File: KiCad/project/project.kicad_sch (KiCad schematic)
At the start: 27 parts, among them P1 TerminalBlock 5P 5.0mm, U1 DRV8313PWPR

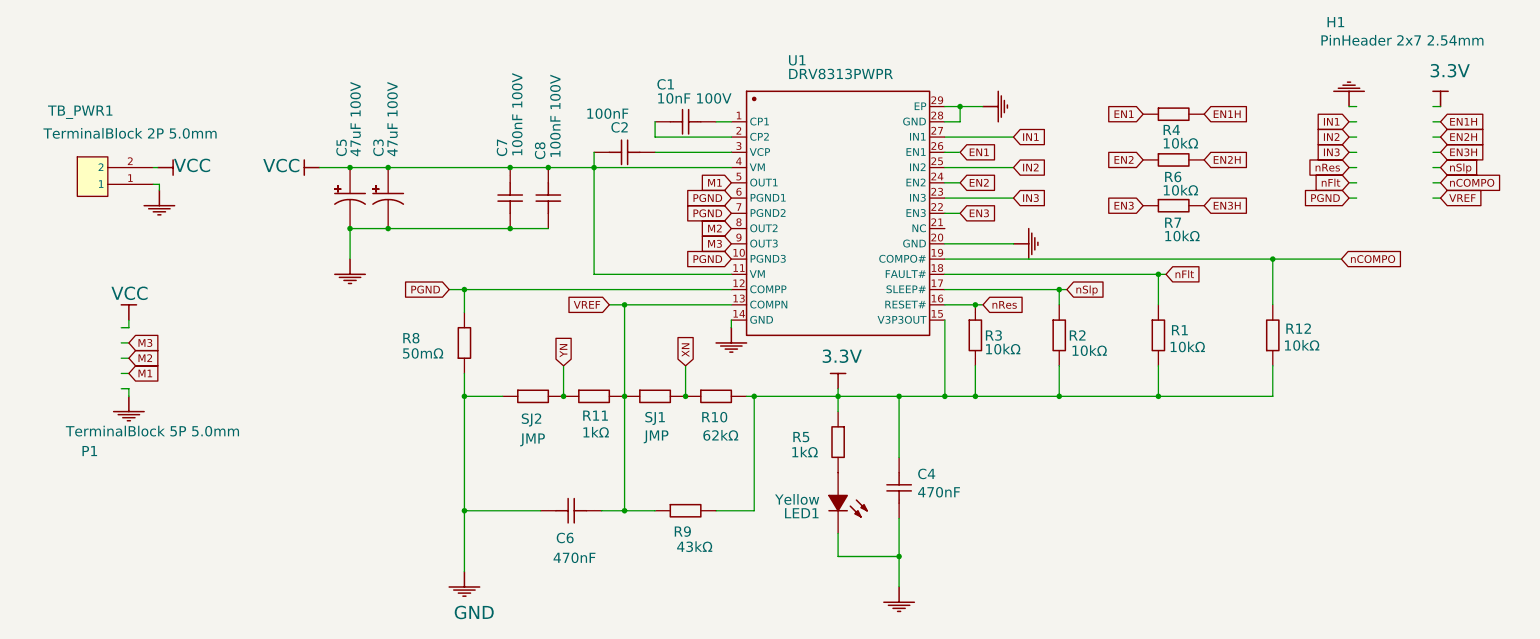
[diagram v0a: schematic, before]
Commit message: Manual layout.
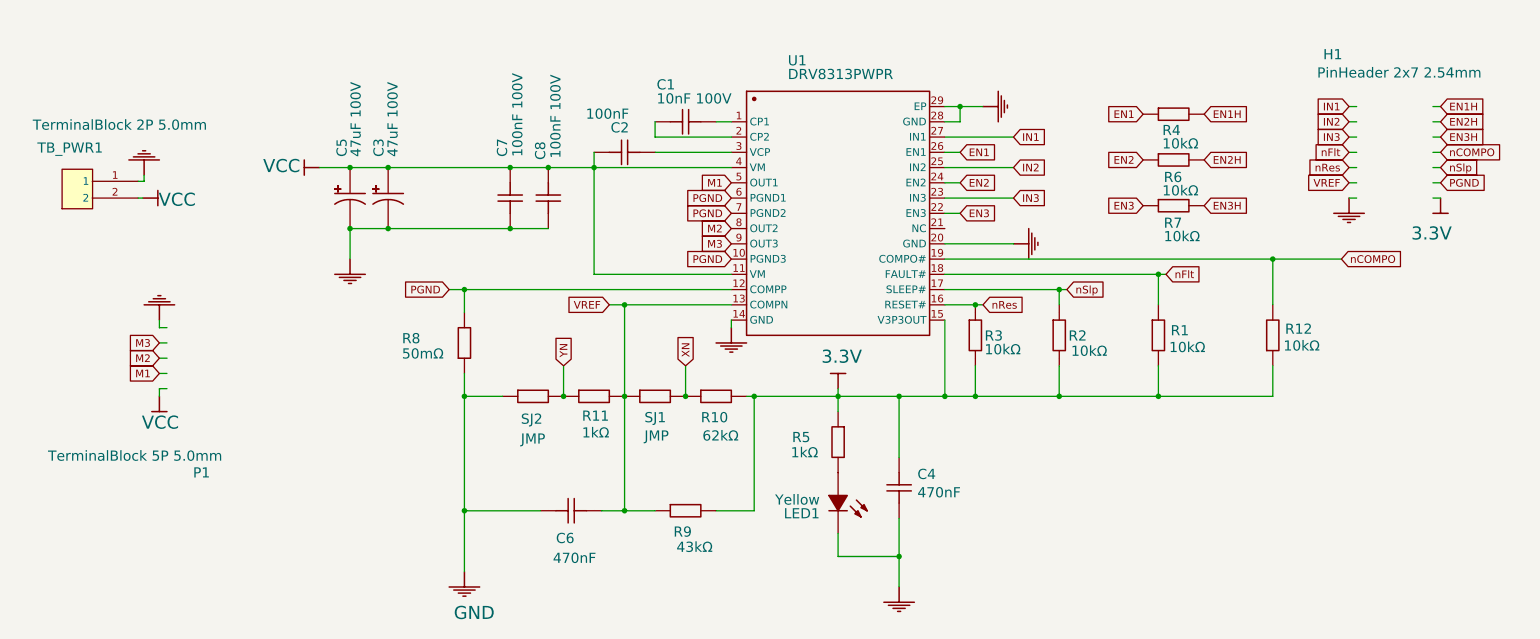
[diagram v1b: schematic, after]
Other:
- moved on the sheet: TB_PWR1
